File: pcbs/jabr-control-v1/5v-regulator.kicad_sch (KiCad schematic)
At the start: 27 parts, among them Q2602 DMN21D2UFB-7B, U1201 TPS259472ARPWR, U1301 MAX20004AFOC/VY+T

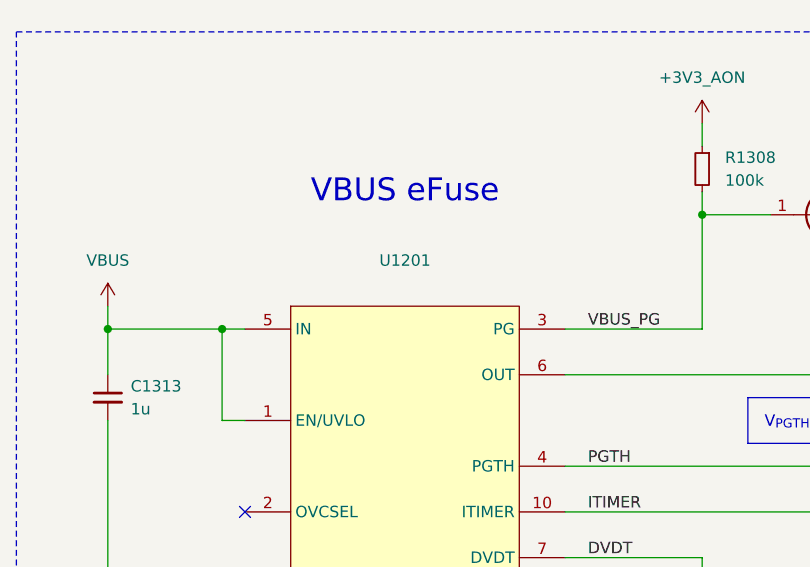
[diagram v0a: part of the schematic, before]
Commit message: Various small updates
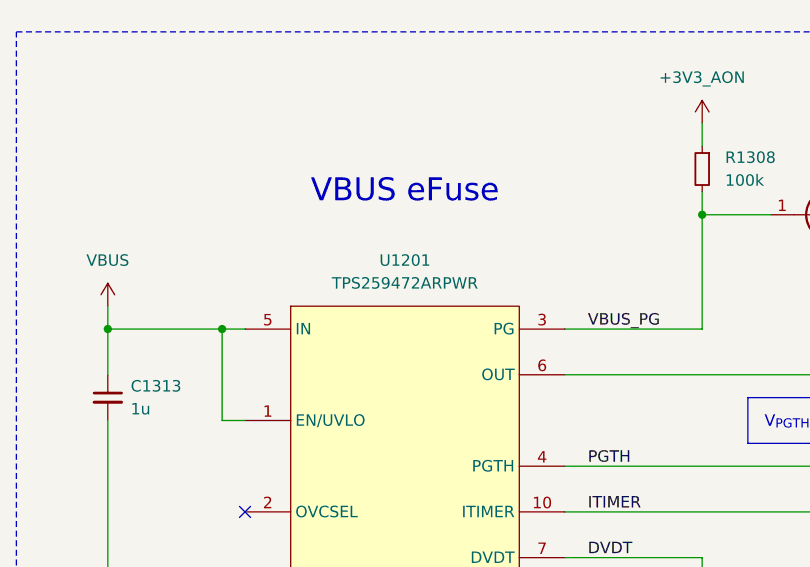
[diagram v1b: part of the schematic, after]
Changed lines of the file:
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@@
 					(size 1.27 1.27)
 				)
-				(hide yes)
 			)
 		)
